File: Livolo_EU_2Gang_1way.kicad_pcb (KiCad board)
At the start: 2 copper layers, 43 x 43 mm, 51 parts, among them IC1 ATMEGA328P, U1 ATSHA204A, U2 RFM69CW, U3 MIC5205-3.3, U4 MCP16301, U5 AT25DF512C

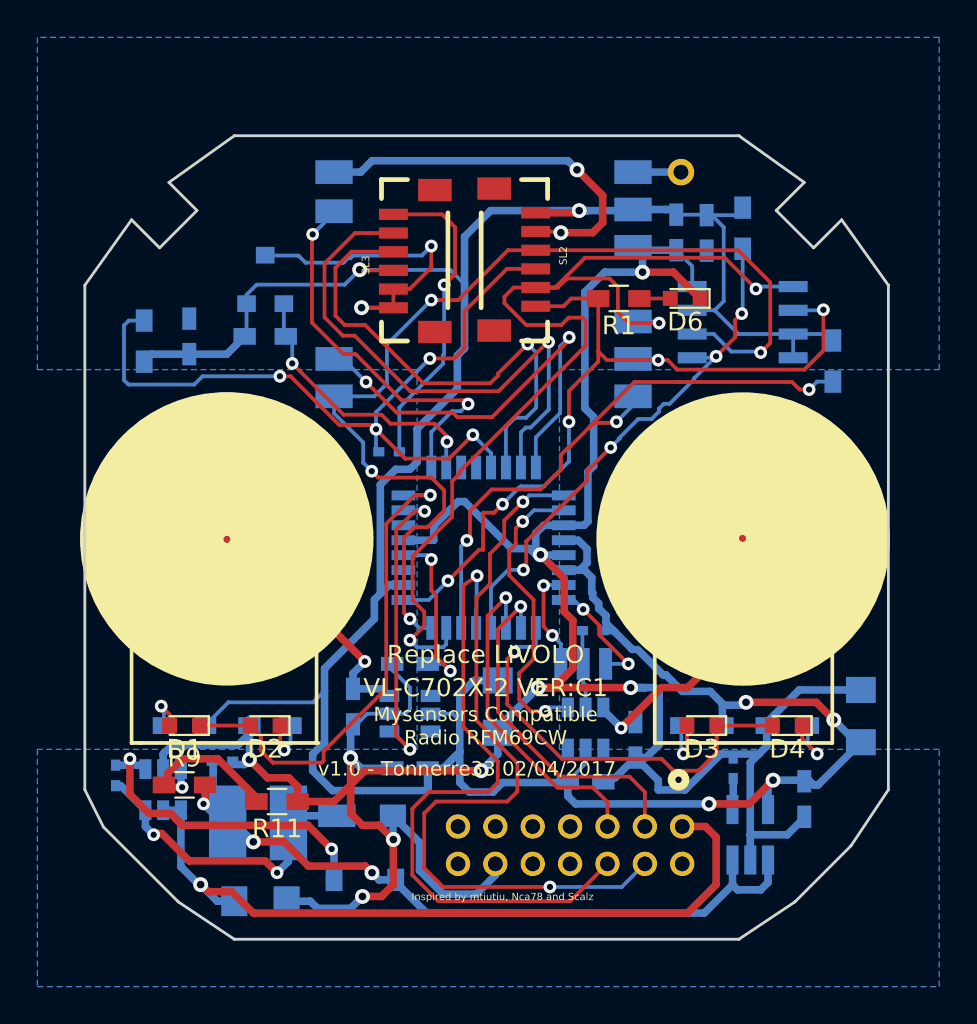
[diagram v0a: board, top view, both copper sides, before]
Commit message: cleaning
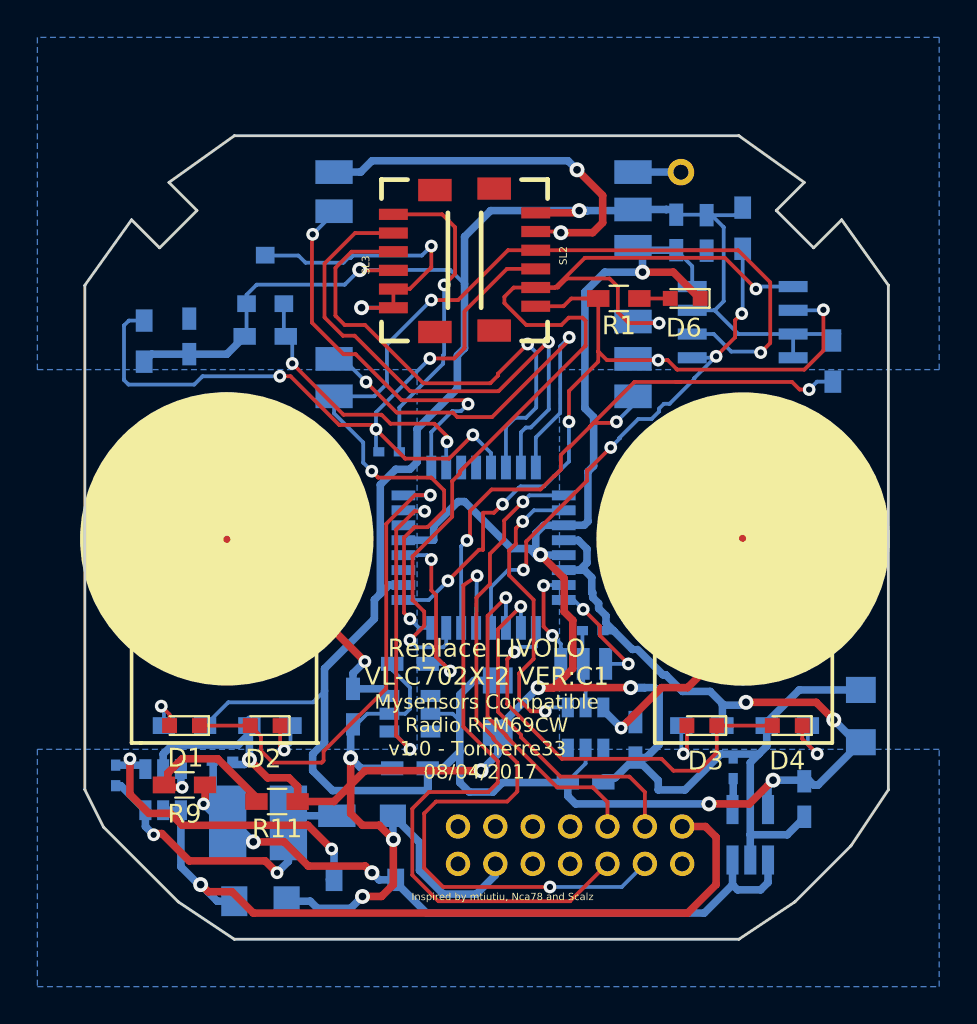
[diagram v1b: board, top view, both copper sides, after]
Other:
- board text added: "v1.0 - Tonnerre33 08/04/2017"
- board text removed: "v1.0 - Tonnerre33 02/04/2017"
